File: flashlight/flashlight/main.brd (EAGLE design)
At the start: 20 x 20 mm, 10 parts

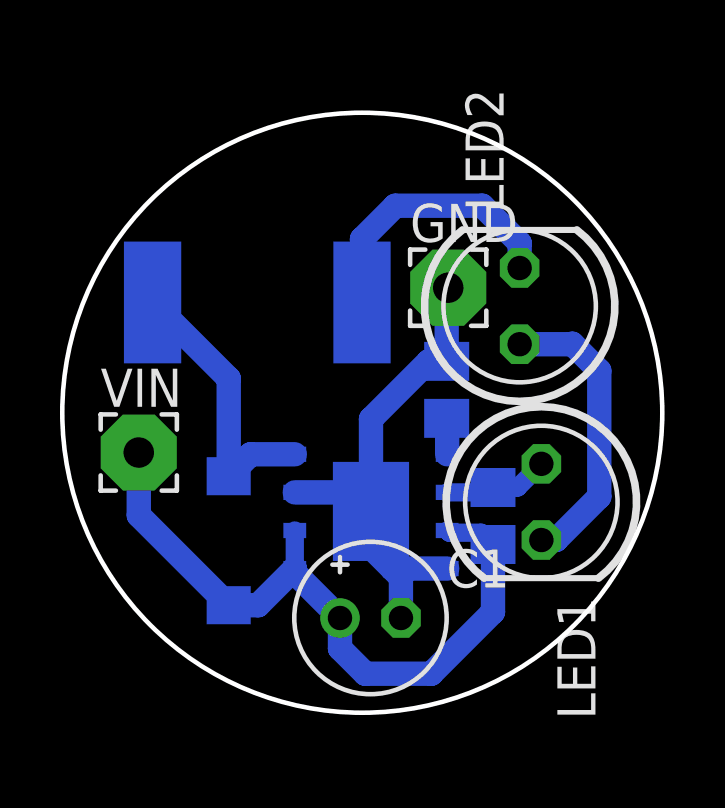
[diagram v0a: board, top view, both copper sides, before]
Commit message: updated project
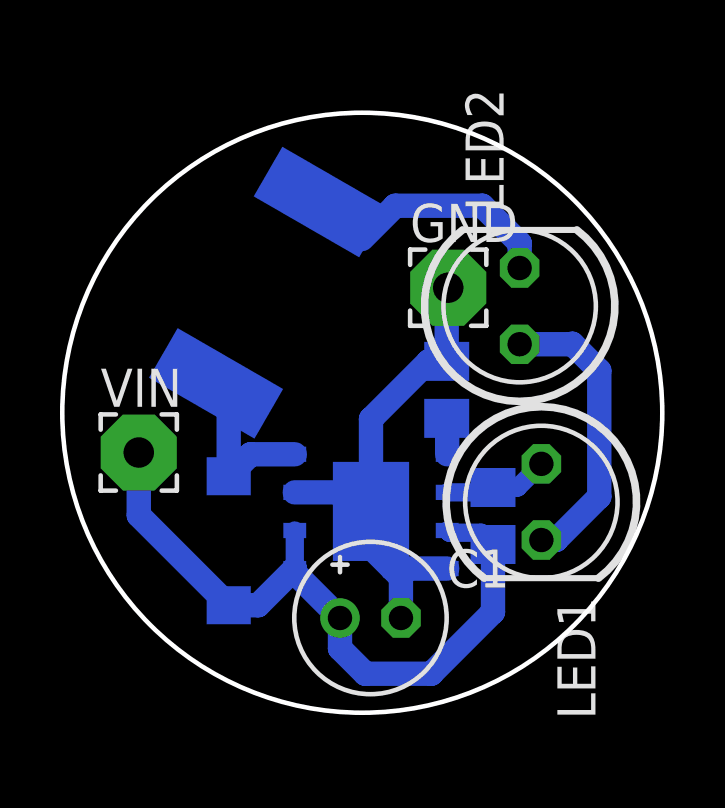
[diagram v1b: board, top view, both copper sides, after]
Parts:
- GND, VIN: device wirepad:2,54/1,0 -> 7_segment_lib:2,54/1,0
- moved U$3 0.49 mm to (-0.73, 6.40), turned to 300 degrees
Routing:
- net N$6: track 9.35 -> 6.01 mm
- net N$7: track 9.18 -> 7.25 mm
